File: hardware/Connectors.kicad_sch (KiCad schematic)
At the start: 21 parts, among them IC12 TLP2367_E, J1 USB_C_Receptacle_USB2.0, J10 M80-5302042, J11 M80-5T10642MC, J14 Conn_01x05, J2 M80-5L10442MC, J3 M300-MV30645M1, J4 M80-5L10442MC, J5 M80-5L10442MC, J6 M80-5L10442MC, J7 M80-5301422, J8 M80-5L10642MC, J9 M80-5L10642MC

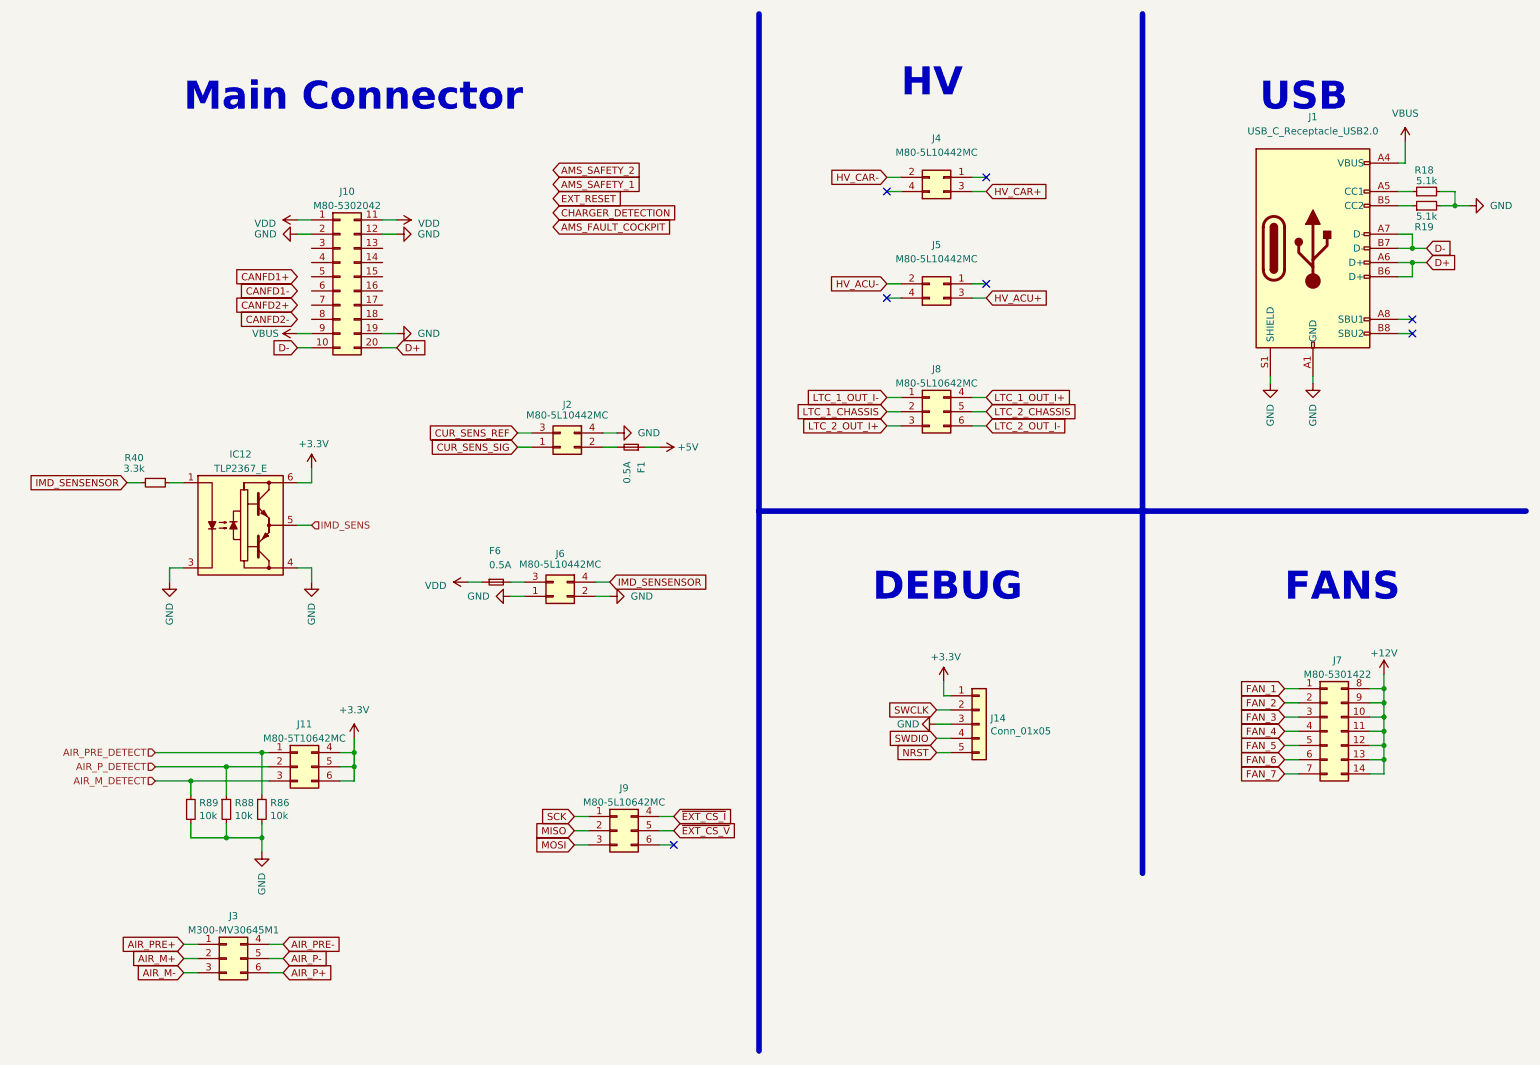
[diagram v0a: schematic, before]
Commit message: further improvements
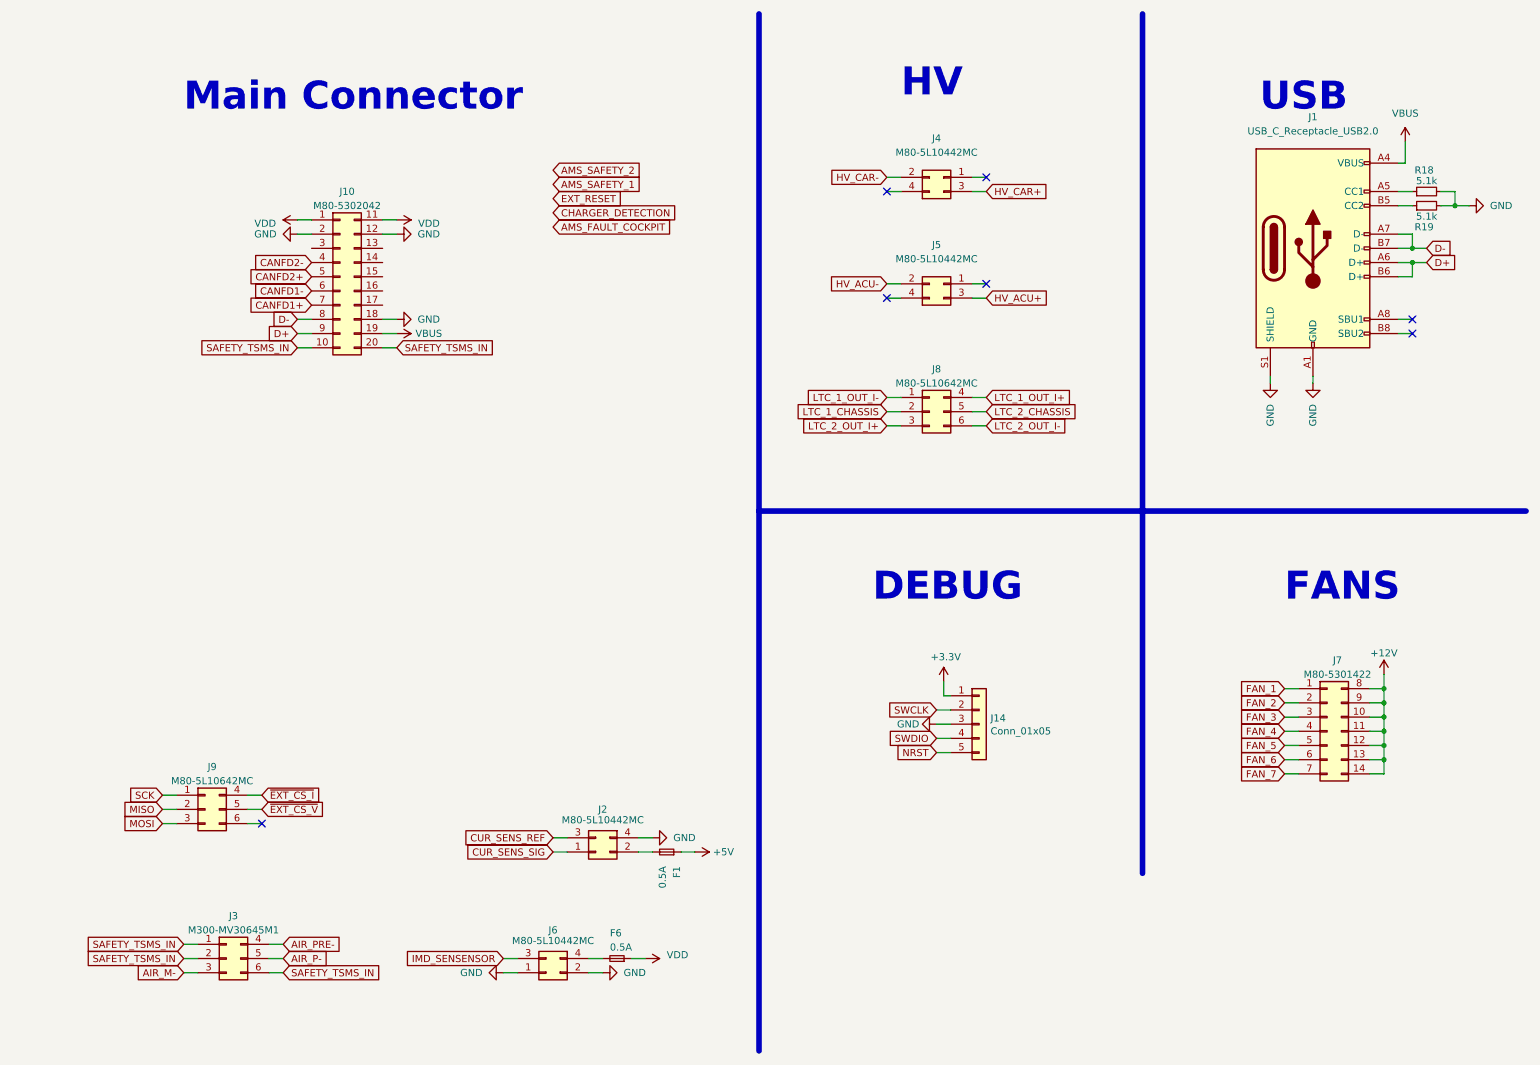
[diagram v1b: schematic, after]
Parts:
- removed IC12: TLP2367_E, TLP2367:SOIC127P700X220-6N, symbol TLP2367_E:TLP2367_E
- removed J11: M80-5T10642MC, M80-5T1062MC:M80-5T106YYMC, symbol M80-5T10642MC:M80-5T10642MC
- removed R40: 3.3k, Resistor_SMD:R_0603_1608Metric, symbol Device:R_Small
- removed R86, R88, R89: 10k, Resistor_SMD:R_0603_1608Metric, symbol Device:R_Small
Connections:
- net AIR_P+ is gone; now on net SAFETY_TSMS_IN: J3.6
- net AIR_PRE+ is gone; now on net SAFETY_TSMS_IN: J3.1
- net CANFD1+: now also J10.7
- net CANFD1-: now also J10.6
- net CANFD2+: now also J10.5
- net CANFD2-: now also J10.4
- net D+: now also J10.9; no longer J10.20
- net D-: now also J10.8; no longer J10.10
- net GND: now also J10.18; no longer J10.19
- net IMD_SENSENSOR: now also J6.3; no longer J6.4
- net VBUS: now also J10.19; no longer J10.9
- net at F6.2: now also J6.4; no longer J6.3
- net AIR_M+ renamed SAFETY_TSMS_IN
- net SAFETY_TSMS_IN: now also J10.10, J10.20
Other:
- moved on the sheet: F1, F6, J2, J6, J9

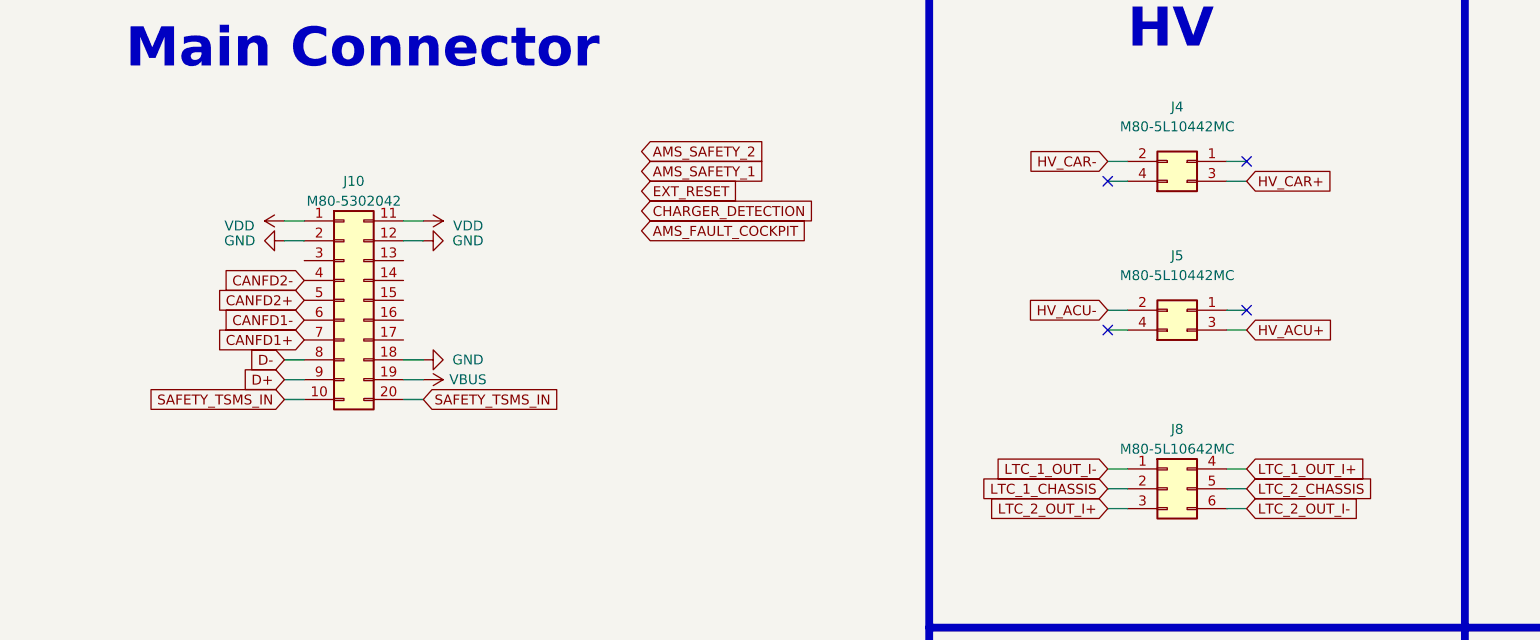
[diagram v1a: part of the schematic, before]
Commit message: PCB routing 50-70% done
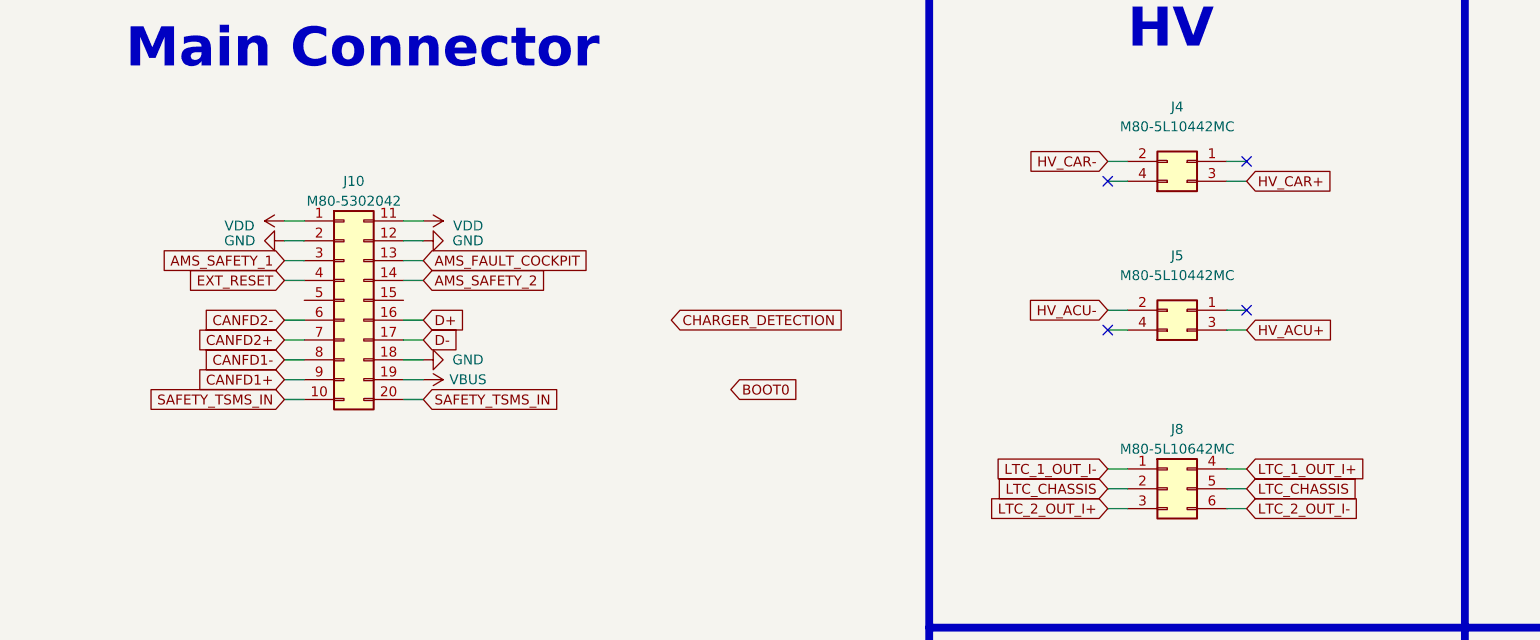
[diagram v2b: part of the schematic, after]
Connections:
- net LTC_2_CHASSIS is gone; now on net LTC_CHASSIS: J8.5
- net AMS_FAULT_COCKPIT: now also J10.13
- net AMS_SAFETY_1: now also J10.3
- net AMS_SAFETY_2: now also J10.14
- net CANFD1+: now also J10.9; no longer J10.7
- net CANFD1-: now also J10.8; no longer J10.6
- net CANFD2+: now also J10.7; no longer J10.5
- net CANFD2-: now also J10.6; no longer J10.4
- net D+: now also J10.16; no longer J10.9
- net D-: now also J10.17; no longer J10.8
- net EXT_RESET: now also J10.4
- net LTC_1_CHASSIS renamed LTC_CHASSIS
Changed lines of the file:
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@@
+    (stroke (width 0) (type default))
+  )
+  (wire (pts (xy 64.77 69.85) (xy 67.31 69.85))
     (stroke (width 0) (type default))
   )
@@
     (stroke (width 0) (type default))
   )
+  (wire (pts (xy 64.77 54.61) (xy 67.31 54.61))
+    (stroke (width 0) (type default))
+  )
   (wire (pts (xy 170.18 63.5) (xy 172.72 63.5))
     (stroke (width 0) (type default))
@@
     (stroke (width 0) (type default))
   )
-  (wire (pts (xy 64.77 69.85) (xy 67.31 69.85))
+  (wire (pts (xy 82.55 64.77) (xy 80.01 64.77))
     (stroke (width 0) (type default))
   )
@@
     (stroke (width 0) (type default))
   )
+  (wire (pts (xy 82.55 57.15) (xy 80.01 57.15))
+    (stroke (width 0) (type default))
+  )
   (wire (pts (xy 59.69 179.07) (xy 62.23 179.07))
     (stroke (width 0) (type default))
@@
     (stroke (width 0) (type default))
   )
+  (wire (pts (xy 64.77 57.15) (xy 67.31 57.15))
+    (stroke (width 0) (type default))
+  )
   (wire (pts (xy 181.61 137.16) (xy 179.07 137.16))
     (stroke (width 0) (type default))
@@
   )
   (wire (pts (xy 261.62 39.37) (xy 262.89 39.37))
+    (stroke (width 0) (type default))
+  )
+  (wire (pts (xy 64.77 62.23) (xy 67.31 62.23))
     (stroke (width 0) (type default))
   )
@@
     (stroke (width 0) (type default))
   )
-  (wire (pts (xy 64.77 67.31) (xy 67.31 67.31))
+  (wire (pts (xy 82.55 62.23) (xy 80.01 62.23))
     (stroke (width 0) (type default))
   )
@@
   )
   (wire (pts (xy 80.01 52.07) (xy 82.55 52.07))
+    (stroke (width 0) (type default))
+  )
+  (wire (pts (xy 80.01 54.61) (xy 82.55 54.61))
     (stroke (width 0) (type default))
   )
@@
     (stroke (width 0) (type default))
   )
+  (wire (pts (xy 64.77 64.77) (xy 67.31 64.77))
+    (stroke (width 0) (type default))
+  )
   (wire (pts (xy 185.42 41.91) (xy 187.96 41.91))
     (stroke (width 0) (type default))
@@
   )
   (wire (pts (xy 243.84 146.05) (xy 241.3 146.05))
+    (stroke (width 0) (type default))
+  )
+  (wire (pts (xy 64.77 67.31) (xy 67.31 67.31))
     (stroke (width 0) (type default))
   )
@@
     )
   )
-  (global_label "CANFD2+" (shape input) (at 67.31 59.69 180) (fields_autoplaced)
-    (effects (font (size 1.27 1.27)) (justify right))
-    (property "Intersheetrefs" "${INTERSHEET_REFS}" (at 56.2288 59.69 0)
+  (global_label "CANFD2+" (shape input) (at 64.77 64.77 180) (fields_autoplaced)
+    (effects (font (size 1.27 1.27)) (justify right))
+    (property "Intersheetrefs" "${INTERSHEET_REFS}" (at 53.6888 64.77 0)
       (effects (font (size 1.27 1.27)) (justify right) hide)
     )
@@
     )
   )
-  (global_label "LTC_1_CHASSIS" (shape input) (at 170.18 83.82 180) (fields_autoplaced)
-    (effects (font (size 1.27 1.27)) (justify right))
-    (property "Intersheetrefs" "${INTERSHEET_REFS}" (at 153.5956 83.82 0)
+  (global_label "LTC_CHASSIS" (shape input) (at 170.18 83.82 180) (fields_autoplaced)
+    (effects (font (size 1.27 1.27)) (justify right))
+    (property "Intersheetrefs" "${INTERSHEET_REFS}" (at 155.7727 83.82 0)
       (effects (font (size 1.27 1.27)) (justify right) hide)
     )
@@
     )
   )
-  (global_label "CANFD1+" (shape input) (at 67.31 64.77 180) (fields_autoplaced)
-    (effects (font (size 1.27 1.27)) (justify right))
-    (property "Intersheetrefs" "${INTERSHEET_REFS}" (at 56.2288 64.77 0)
+  (global_label "CANFD1+" (shape input) (at 64.77 69.85 180) (fields_autoplaced)
+    (effects (font (size 1.27 1.27)) (justify right))
+    (property "Intersheetrefs" "${INTERSHEET_REFS}" (at 53.6888 69.85 0)
       (effects (font (size 1.27 1.27)) (justify right) hide)
     )
@@
     )
   )
-  (global_label "CANFD1-" (shape input) (at 67.31 62.23 180) (fields_autoplaced)
-    (effects (font (size 1.27 1.27)) (justify right))
-    (property "Intersheetrefs" "${INTERSHEET_REFS}" (at 56.2288 62.23 0)
+  (global_label "CANFD1-" (shape input) (at 64.77 67.31 180) (fields_autoplaced)
+    (effects (font (size 1.27 1.27)) (justify right))
+    (property "Intersheetrefs" "${INTERSHEET_REFS}" (at 53.6888 67.31 0)
       (effects (font (size 1.27 1.27)) (justify right) hide)
     )
@@
     )
   )
-  (global_label "EXT_RESET" (shape input) (at 110.49 45.72 0) (fields_autoplaced)
-    (effects (font (size 1.27 1.27)) (justify left))
-    (property "Intersheetrefs" "${INTERSHEET_REFS}" (at 122.7804 45.72 0)
-      (effects (font (size 1.27 1.27)) (justify left) hide)
-    )
-  )
-  (global_label "AMS_FAULT_COCKPIT" (shape input) (at 110.49 50.8 0) (fields_autoplaced)
-    (effects (font (size 1.27 1.27)) (justify left))
-    (property "Intersheetrefs" "${INTERSHEET_REFS}" (at 131.9126 50.8 0)
+  (global_label "EXT_RESET" (shape input) (at 64.77 57.15 180) (fields_autoplaced)
+    (effects (font (size 1.27 1.27)) (justify right))
+    (property "Intersheetrefs" "${INTERSHEET_REFS}" (at 52.4796 57.15 0)
+      (effects (font (size 1.27 1.27)) (justify right) hide)
+    )
+  )
+  (global_label "AMS_FAULT_COCKPIT" (shape input) (at 82.55 54.61 0) (fields_autoplaced)
+    (effects (font (size 1.27 1.27)) (justify left))
+    (property "Intersheetrefs" "${INTERSHEET_REFS}" (at 103.9726 54.61 0)
       (effects (font (size 1.27 1.27)) (justify left) hide)
     )
@@
     )
   )
-  (global_label "CHARGER_DETECTION" (shape input) (at 110.49 48.26 0) (fields_autoplaced)
-    (effects (font (size 1.27 1.27)) (justify left))
-    (property "Intersheetrefs" "${INTERSHEET_REFS}" (at 132.3963 48.26 0)
+  (global_label "CHARGER_DETECTION" (shape input) (at 114.3 62.23 0) (fields_autoplaced)
+    (effects (font (size 1.27 1.27)) (justify left))
+    (property "Intersheetrefs" "${INTERSHEET_REFS}" (at 136.2063 62.23 0)
       (effects (font (size 1.27 1.27)) (justify left) hide)
     )
@@
     )
   )
-  (global_label "AMS_SAFETY_2" (shape input) (at 110.49 40.64 0) (fields_autoplaced)
-    (effects (font (size 1.27 1.27)) (justify left))
-    (property "Intersheetrefs" "${INTERSHEET_REFS}" (at 126.2277 40.64 0)
+  (global_label "AMS_SAFETY_2" (shape input) (at 82.55 57.15 0) (fields_autoplaced)
+    (effects (font (size 1.27 1.27)) (justify left))
+    (property "Intersheetrefs" "${INTERSHEET_REFS}" (at 98.2877 57.15 0)
       (effects (font (size 1.27 1.27)) (justify left) hide)
     )
@@
     )
   )
-  (global_label "AMS_SAFETY_1" (shape input) (at 110.49 43.18 0) (fields_autoplaced)
-    (effects (font (size 1.27 1.27)) (justify left))
-    (property "Intersheetrefs" "${INTERSHEET_REFS}" (at 126.2277 43.18 0)
-      (effects (font (size 1.27 1.27)) (justify left) hide)
-    )
-  )
-  (global_label "D+" (shape input) (at 64.77 69.85 180) (fields_autoplaced)
-    (effects (font (size 1.27 1.27)) (justify right))
-    (property "Intersheetrefs" "${INTERSHEET_REFS}" (at 59.676 69.85 0)
-      (effects (font (size 1.27 1.27)) (justify right) hide)
+  (global_label "AMS_SAFETY_1" (shape input) (at 64.77 54.61 180) (fields_autoplaced)
+    (effects (font (size 1.27 1.27)) (justify right))
+    (property "Intersheetrefs" "${INTERSHEET_REFS}" (at 49.0323 54.61 0)
+      (effects (font (size 1.27 1.27)) (justify right) hide)
+    )
+  )
+  (global_label "D+" (shape input) (at 82.55 62.23 0) (fields_autoplaced)
+    (effects (font (size 1.27 1.27)) (justify left))
+    (property "Intersheetrefs" "${INTERSHEET_REFS}" (at 87.644 62.23 0)
+      (effects (font (size 1.27 1.27)) (justify left) hide)
     )
   )
@@
     )
   )
+  (global_label "BOOT0" (shape input) (at 121.92 71.12 0) (fields_autoplaced)
+    (effects (font (size 1.27 1.27)) (justify left))
+    (property "Intersheetrefs" "${INTERSHEET_REFS}" (at 26.67 -26.67 0)
+      (effects (font (size 1.27 1.27)) hide)
+    )
+  )
   (global_label "D+" (shape input) (at 266.7 57.15 0) (fields_autoplaced)
     (effects (font (size 1.27 1.27)) (justify left))
@@
     )
   )
-  (global_label "CANFD2-" (shape input) (at 67.31 57.15 180) (fields_autoplaced)
-    (effects (font (size 1.27 1.27)) (justify right))
-    (property "Intersheetrefs" "${INTERSHEET_REFS}" (at 56.2288 57.15 0)
+  (global_label "CANFD2-" (shape input) (at 64.77 62.23 180) (fields_autoplaced)
+    (effects (font (size 1.27 1.27)) (justify right))
+    (property "Intersheetrefs" "${INTERSHEET_REFS}" (at 53.6888 62.23 0)
       (effects (font (size 1.27 1.27)) (justify right) hide)
     )
@@
     )
   )
+  (global_label "LTC_CHASSIS" (shape input) (at 187.96 83.82 0) (fields_autoplaced)
+    (effects (font (size 1.27 1.27)) (justify left))
+    (property "Intersheetrefs" "${INTERSHEET_REFS}" (at 202.3673 83.82 0)
+      (effects (font (size 1.27 1.27)) (justify left) hide)
+    )
+  )
   (global_label "LTC_1_OUT_I+" (shape input) (at 187.96 81.28 0) (fields_autoplaced)
     (effects (font (size 1.27 1.27)) (justify left))
@@
     )
   )
-  (global_label "D-" (shape input) (at 64.77 67.31 180) (fields_autoplaced)
-    (effects (font (size 1.27 1.27)) (justify right))
-    (property "Intersheetrefs" "${INTERSHEET_REFS}" (at 59.676 67.31 0)
-      (effects (font (size 1.27 1.27)) (justify right) hide)
-    )
-  )
-  (global_label "LTC_2_CHASSIS" (shape input) (at 187.96 83.82 0) (fields_autoplaced)
-    (effects (font (size 1.27 1.27)) (justify left))
-    (property "Intersheetrefs" "${INTERSHEET_REFS}" (at 204.5444 83.82 0)
-      (effects (font (size 1.27 1.27)) (justify left) hide)
-    )
+  (global_label "D-" (shape input) (at 82.55 64.77 0) (fields_autoplaced)
+    (effects (font (size 1.27 1.27)) (justify left))
+    (property "Intersheetrefs" "${INTERSHEET_REFS}" (at 87.644 64.77 0)
+      (effects (font (size 1.27 1.27)) (justify left) hide)
+    )
